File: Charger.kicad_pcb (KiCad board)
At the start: 2 copper layers, 12 parts, among them J1 Input, J2 USB-A-S-X-X-SM2, U1 LT1085-5.0

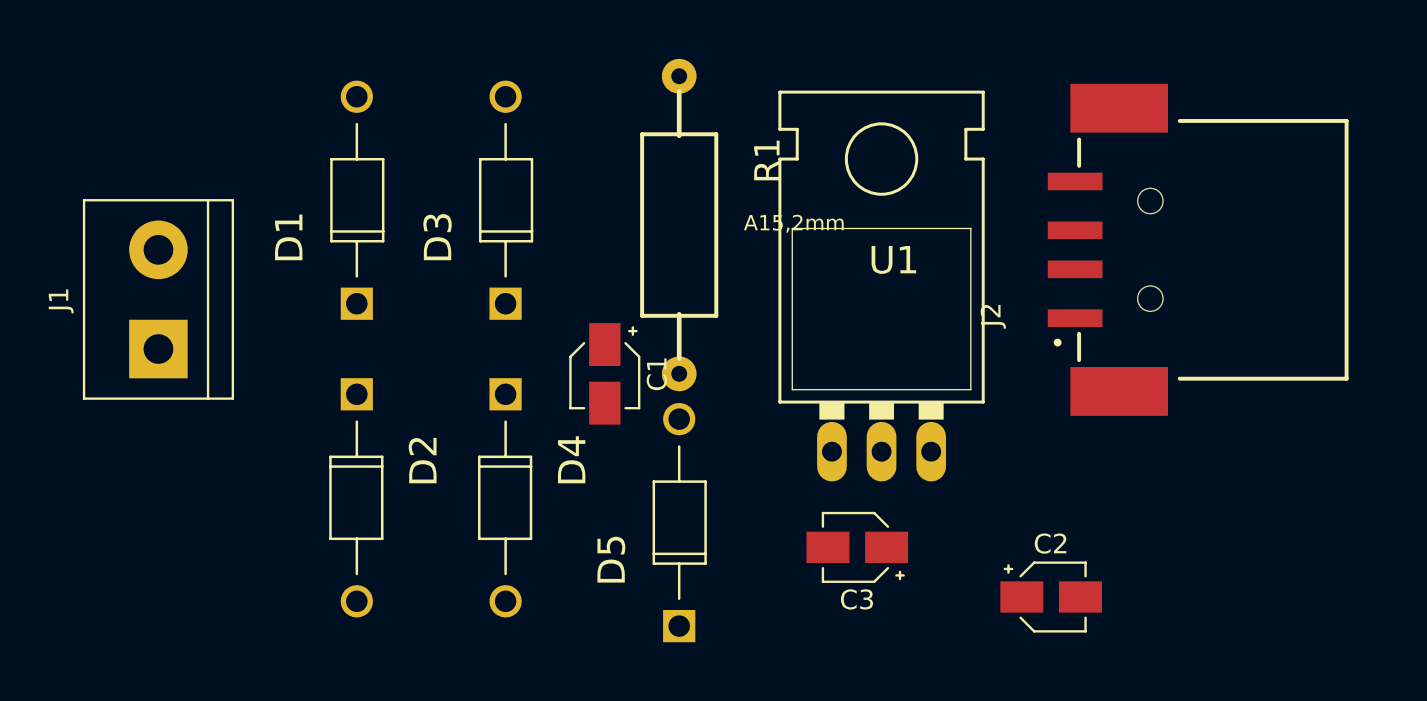
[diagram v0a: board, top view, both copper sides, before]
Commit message: Update Charger.kicad_pcb
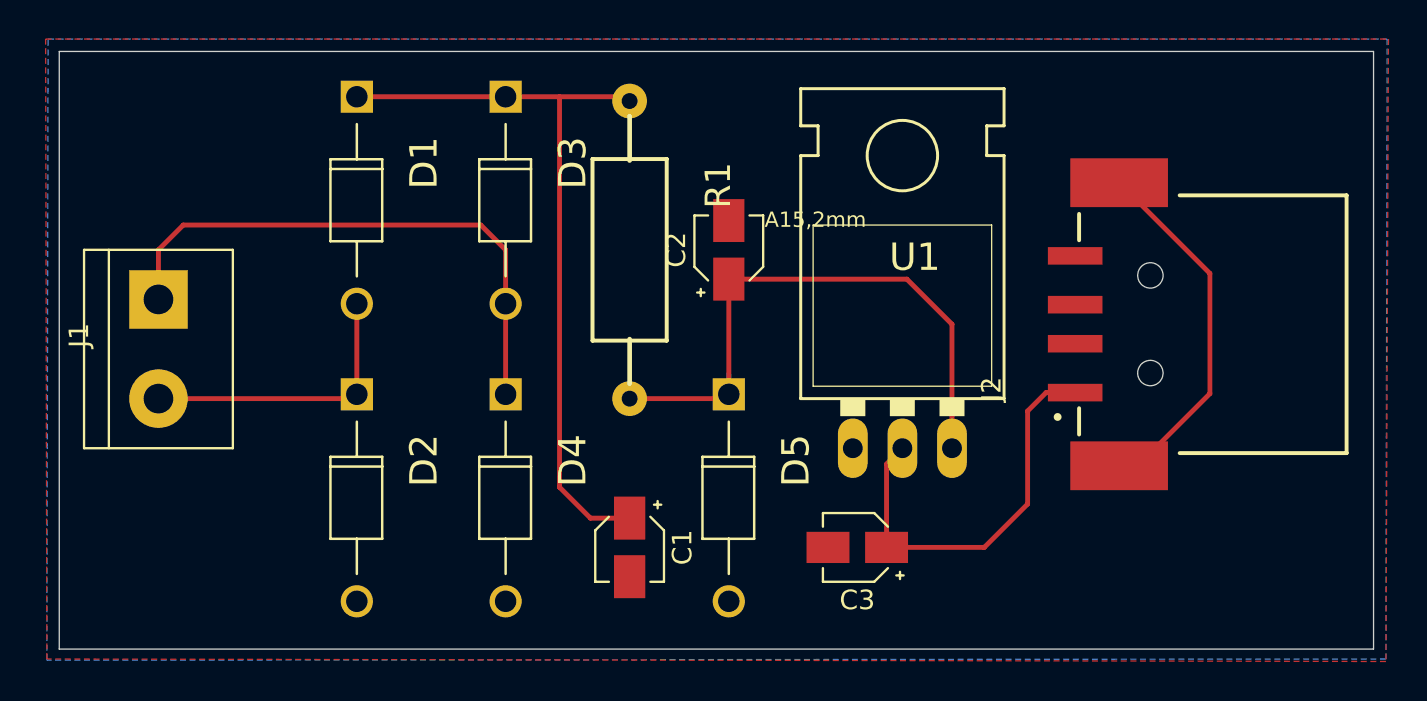
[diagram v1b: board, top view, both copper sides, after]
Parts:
- moved C2 24.3 mm to (462.3, 1047.8), turned to 90 degrees
- moved C1 8.98 mm to (457.2, 1063.0)
- moved J2 3.81 mm to (483.9, 1051.6)
- moved R1 2.84 mm to (457.2, 1047.8)
- moved D5 2.84 mm to (462.3, 1060.5), turned to 270 degrees
- moved J1 2.54 mm to (433.1, 1050.3), turned to 270 degrees
- moved U1 1.08 mm to (471.2, 1054.1)
- turned D1 to 270 degrees
- turned D3 to 270 degrees
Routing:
- net Net-(C1-Pad1): track 0.00 -> 38.3 mm
- net Net-(C2-Pad1): track 0.00 -> 30.9 mm
- net +: track 0.00 -> 28.8 mm
- net Vout: track 0.00 -> 21.2 mm
- net Net-(J2-PadS1): track 0.00 -> 19.1 mm
- net -: track 0.00 -> 14.9 mm
- added copper zone on B.Cu, net (none)
- added copper zone on F.Cu, net gnd
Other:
- board outline added: 67.3 x 30.6 mm
- board text added: "1N4005"
- board text added: "20 ohm"
- board text added: "BZX85C10"
- board text added: "LT1085-5.0"
- board text added: "USB"
- board text added: "input"
